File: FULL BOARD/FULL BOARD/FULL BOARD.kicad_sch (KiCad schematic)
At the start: 113 parts, among them IC1 TAS5760LDAP, J1 PJ-036AH-SMT-TR, J2 Micro_SD_Card, J3 B2B-PH-K-S, J4 5019514000, J5 61201021621, J6 B2B-PH-K-S, SW1 PTS645SK50SMTR92LFS, U1 LD1117S33TR_SOT223, U2 STM32H743VITx, Y1 ABLS7M2-16.000MHZ-D-2Y-T

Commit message: changed reset footprint
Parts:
- SW1: footprint push button custom:SW4_PTS645SK50SMTR92LFS_CNK -> Reset Switch:SW_PTS645SK50SMTR92LFS
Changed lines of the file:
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@@
 			)
 		)
-		(property "Footprint" "push button custom:SW4_PTS645SK50SMTR92LFS_CNK"
+		(property "Footprint" "Reset Switch:SW_PTS645SK50SMTR92LFS"
 			(at 34.29 142.24 0)
 			(effects

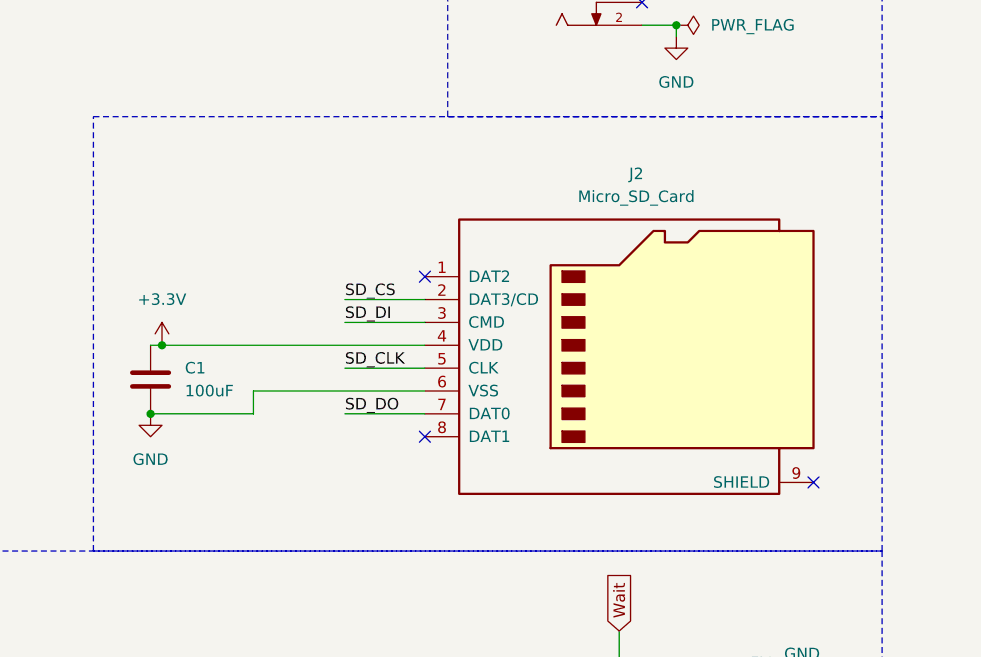
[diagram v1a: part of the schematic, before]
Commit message: change SD
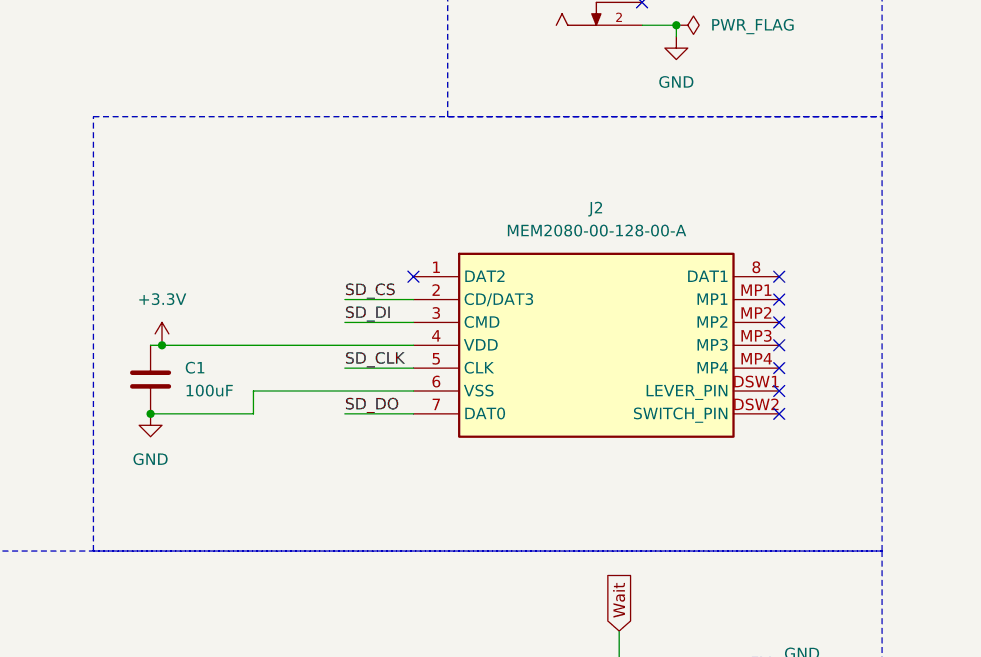
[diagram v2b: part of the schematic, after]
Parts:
- removed J2: Micro_SD_Card, Connector_Card:microSD_HC_Molex_47219-2001, symbol Connector:Micro_SD_Card
- added J2: MEM2080-00-128-00-A, MEM20800012800A, symbol Second SD Card:MEM2080-00-128-00-A
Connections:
- net +3.3V: now also J2.4 (VDD)
- net GND: now also J2.6 (VSS)
- net SD_CLK: now also J2.5 (CLK)
- net SD_CS: now also J2.2 (CD/DAT3)
- net SD_DI: now also J2.3 (CMD)
- net SD_DO: now also J2.7 (DAT0)
- no-connect marks 94 -> 99
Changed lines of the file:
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@@
 	)
 	(no_connect
-		(at 30.48 304.8)
+		(at 322.58 152.4)
 	)
 	(no_connect
-		(at 283.21 154.94)
+		(at 30.48 304.8)
 	)
 	(no_connect
@@
 	)
 	(no_connect
+		(at 322.58 144.78)
+	)
+	(no_connect
 		(at 128.27 199.39)
 	)
@@
 	)
 	(no_connect
-		(at 283.21 137.16)
+		(at 281.94 137.16)
+	)
+	(no_connect
+		(at 322.58 139.7)
 	)
 	(no_connect
@@
 	)
 	(no_connect
+		(at 322.58 137.16)
+	)
+	(no_connect
 		(at 269.24 190.5)
 	)
@@
 	)
 	(no_connect
+		(at 322.58 149.86)
+	)
+	(no_connect
 		(at 138.43 135.89)
 	)
@@
 	)
 	(no_connect
+		(at 322.58 147.32)
+	)
+	(no_connect
 		(at 181.61 163.83)
 	)
@@
 	)
 	(no_connect
+		(at 322.58 142.24)
+	)
+	(no_connect
 		(at 292.1 190.5)
 	)
@@
 	)
 	(no_connect
-		(at 326.39 160.02)
-	)
-	(no_connect
 		(at 138.43 168.91)
 	)
@@
 	(wire
 		(pts
-			(xy 274.32 139.7) (xy 283.21 139.7)
+			(xy 274.32 139.7) (xy 281.94 139.7)
 		)
 		(stroke
@@
 	(wire
 		(pts
-			(xy 274.32 147.32) (xy 283.21 147.32)
+			(xy 274.32 147.32) (xy 281.94 147.32)
 		)
 		(stroke
@@
 	(wire
 		(pts
-			(xy 264.16 149.86) (xy 283.21 149.86)
+			(xy 264.16 149.86) (xy 281.94 149.86)
 		)
 		(stroke
@@
 	(wire
 		(pts
-			(xy 274.32 152.4) (xy 283.21 152.4)
+			(xy 274.32 152.4) (xy 281.94 152.4)
 		)
 		(stroke
@@
 	(wire
 		(pts
-			(xy 254 144.78) (xy 283.21 144.78)
+			(xy 254 144.78) (xy 281.94 144.78)
 		)
 		(stroke
@@
 	(wire
 		(pts
-			(xy 274.32 142.24) (xy 283.21 142.24)
+			(xy 274.32 142.24) (xy 281.94 142.24)
 		)
 		(stroke
@@
 	)
 	(symbol
+		(lib_id "Second SD Card:MEM2080-00-128-00-A")
+		(at 281.94 137.16 0)
+		(unit 1)
+		(exclude_from_sim no)
+		(in_bom yes)
+		(on_board yes)
+		(dnp no)
+		(fields_autoplaced yes)
+		(property "Reference" "J2"
+			(at 302.26 129.54 0)
+			(effects
+				(font
+					(size 1.27 1.27)
+				)
+			)
+		)
+		(property "Value" "MEM2080-00-128-00-A"
+			(at 302.26 132.08 0)
+			(effects
+				(font
+					(size 1.27 1.27)
+				)
+			)
+		)
+		(property "Footprint" "MEM20800012800A"
+			(at 318.77 232.08 0)
+			(effects
+				(font
+					(size 1.27 1.27)
+				)
+				(justify left top)
+				(hide yes)
+			)
+		)
+		(property "Datasheet" "https://gct.co/files/drawings/mem2080.pdf?v=a9dd5643-7d1c-4e6b-bf46-1b82bcb8595f"
+			(at 318.77 332.08 0)
+			(effects
+				(font
+					(size 1.27 1.27)
+				)
+				(justify left top)
+				(hide yes)
+			)
+		)
+		(property "Description" "Memory Card Connectors Micro SD, Push Push, SMT, Card Entry Normal, 1.28 mm profile"
+			(at 281.94 137.16 0)
+			(effects
+				(font
+					(size 1.27 1.27)
+				)
+				(hide yes)
+			)
+		)
+		(property "Height" "1.48"
+			(at 318.77 532.08 0)
+			(effects
+				(font
+					(size 1.27 1.27)
+				)
+				(justify left top)
+				(hide yes)
+			)
+		)
+		(property "Mouser Part Number" "640-MEM2080-0012800A"
+			(at 318.77 632.08 0)
+			(effects
+				(font
+					(size 1.27 1.27)
+				)
+				(justify left top)
+				(hide yes)
+			)
+		)
+		(property "Mouser Price/Stock" "https://www.mouser.co.uk/ProductDetail/GCT/MEM2080-00-128-00-A?qs=vvQtp7zwQdPJXzpf1SnYug%3D%3D"
+			(at 318.77 732.08 0)
+			(effects
+				(font
+					(size 1.27 1.27)
+				)
+				(justify left top)
+				(hide yes)
+			)
+		)
+		(property "Manufacturer_Name" "GCT (GLOBAL CONNECTOR TECHNOLOGY)"
+			(at 318.77 832.08 0)
+			(effects
+				(font
+					(size 1.27 1.27)
+				)
+				(justify left top)
+				(hide yes)
+			)
+		)
+		(property "Manufacturer_Part_Number" "MEM2080-00-128-00-A"
+			(at 318.77 932.08 0)
+			(effects
+				(font
+					(size 1.27 1.27)
+				)
+				(justify left top)
+				(hide yes)
+			)
+		)
+		(pin "4"
+		)
+		(pin "6"
+		)
+		(pin "7"
+		)
+		(pin "MP1"
+		)
+		(pin "MP3"
+		)
+		(pin "MP2"
+		)
+		(pin "DSW1"
+		)
+		(pin "8"
+		)
+		(pin "1"
+		)
+		(pin "3"
+		)
+		(pin "DSW2"
+		)
+		(pin "MP4"
+		)
+		(pin "2"
+		)
+		(pin "5"
+		)
+		(instances
+			(project ""
+				(path "/df550598-5349-47af-a3f3-2a2a958bedd4"
+					(reference "J2")
+					(unit 1)
+				)
+			)
+		)
+	)
+	(symbol
 		(lib_id "Device:C")
 		(at 31.75 113.03 0)
@@
 					(unit 1)
 				)
-			)
-		)
-	)
-	(symbol
-		(lib_id "Connector:Micro_SD_Card")
-		(at 306.07 144.78 0)
-		(unit 1)
-		(exclude_from_sim no)
-		(in_bom yes)
-		(on_board yes)
-		(dnp no)
-		(fields_autoplaced yes)
-		(property "Reference" "J2"
-			(at 306.705 125.73 0)
-			(effects
-				(font
-					(size 1.27 1.27)
-				)
-			)
-		)
-		(property "Value" "Micro_SD_Card"
-			(at 306.705 128.27 0)
-			(effects
-				(font
-					(size 1.27 1.27)
-				)
-			)
-		)
-		(property "Footprint" "Connector_Card:microSD_HC_Molex_47219-2001"
-			(at 335.28 137.16 0)
-			(effects
-				(font
-					(size 1.27 1.27)
-				)
-				(hide yes)
-			)
-		)
-		(property "Datasheet" "http://katalog.we-online.de/em/datasheet/693072010801.pdf"
-			(at 306.07 144.78 0)
-			(effects
-				(font
-					(size 1.27 1.27)
-				)
-				(hide yes)
-			)
-		)
-		(property "Description" "Micro SD Card Socket"
-			(at 306.07 144.78 0)
-			(effects
-				(font
-					(size 1.27 1.27)
-				)
-				(hide yes)
-			)
-		)
-		(pin "3"
-		)
-		(pin "2"
-		)
-		(pin "9"
-		)
-		(pin "8"
-		)
-		(pin "5"
-		)
-		(pin "1"
-		)
-		(pin "4"
-		)
-		(pin "6"
-		)
-		(pin "7"
-		)
-		(instances
-			(project ""
-				(path "/df550598-5349-47af-a3f3-2a2a958bedd4"
-					(reference "J2")
-					(unit 1)
-				)
